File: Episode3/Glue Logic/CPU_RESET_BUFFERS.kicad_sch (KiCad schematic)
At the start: 26 parts, among them SW1 RST SW, U1 HD63C09P, U2 MIC1232, U3 74HCT541, U4 74HCT541, U5 74HCT245, U6 74HCT125

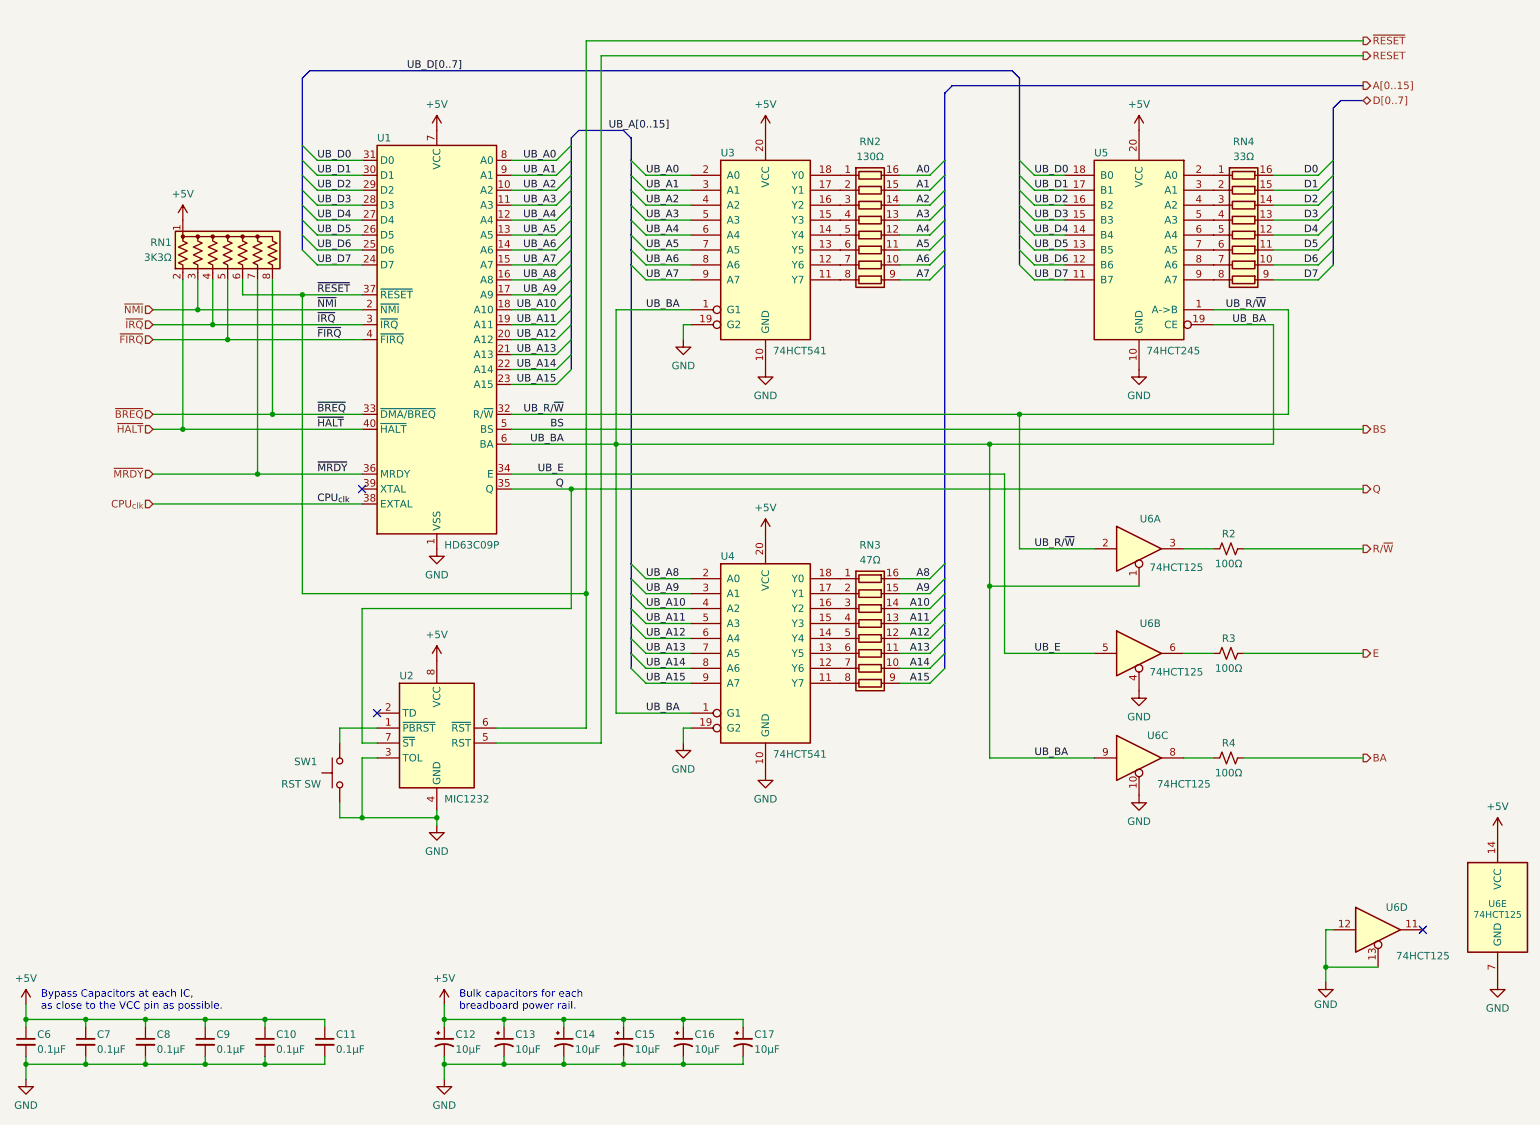
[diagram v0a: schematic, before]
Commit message: Exploited every last macrocells I could.
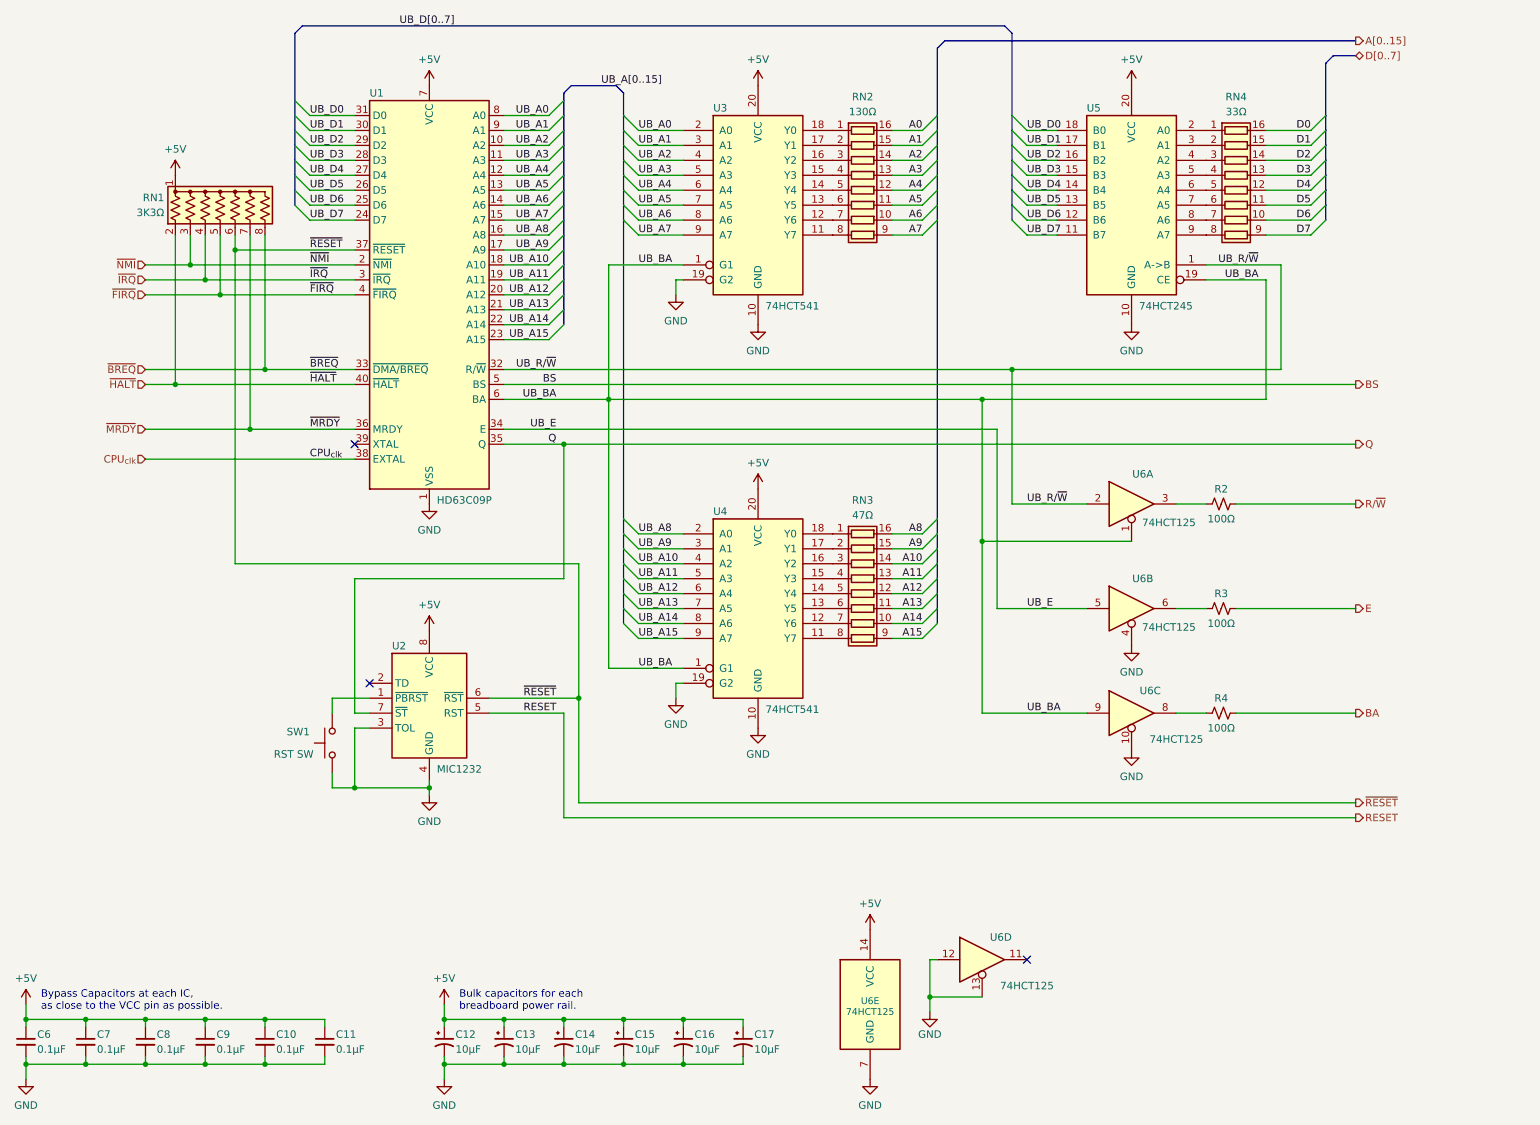
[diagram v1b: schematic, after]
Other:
- moved on the sheet: R2, R3, R4, RN1, RN2, RN3, RN4, SW1, U1, U2, U3, U4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
